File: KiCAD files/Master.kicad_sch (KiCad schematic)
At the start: 24 parts, among them SW1 EG1271A, SW2 EG1271A, SW3 EG1271A, SW4 EG1271A, U4 NUCLEO64-F446RE

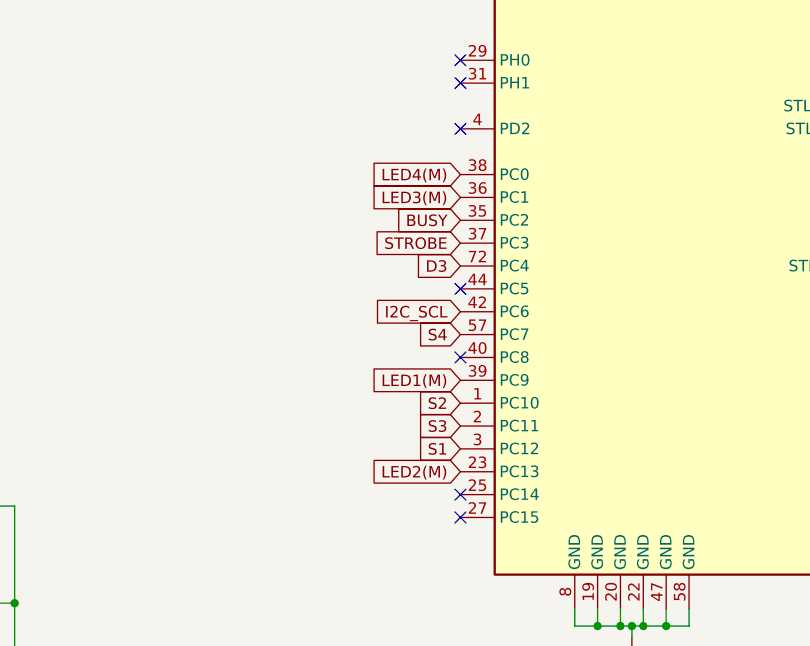
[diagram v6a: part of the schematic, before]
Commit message: update
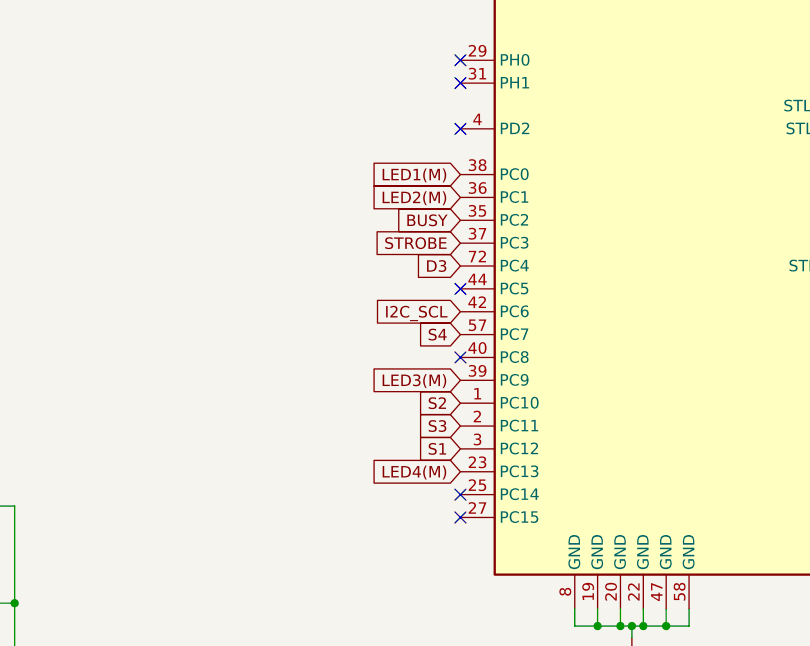
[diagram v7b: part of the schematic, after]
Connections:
- net LED1(M): now also U4.38 (PC0); no longer U4.39 (PC9)
- net LED2(M): now also U4.36 (PC1); no longer U4.23 (PC13)
- net LED3(M): now also U4.39 (PC9); no longer U4.36 (PC1)
- net LED4(M): now also U4.23 (PC13); no longer U4.38 (PC0)
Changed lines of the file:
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@@
     )
   )
-  (global_label "LED1(M)" (shape input) (at 113.665 116.84 180) (fields_autoplaced)
+  (global_label "LED1(M)" (shape input) (at 113.665 93.98 180) (fields_autoplaced)
     (effects (font (size 1.27 1.27)) (justify right))
-    (property "Intersheetrefs" "${INTERSHEET_REFS}" (at 102.8784 116.84 0)
+    (property "Intersheetrefs" "${INTERSHEET_REFS}" (at 102.8784 93.98 0)
       (effects (font (size 1.27 1.27)) (justify right) hide)
     )
   )
-  (global_label "LED3(M)" (shape input) (at 113.665 96.52 180) (fields_autoplaced)
+  (global_label "LED3(M)" (shape input) (at 113.665 116.84 180) (fields_autoplaced)
     (effects (font (size 1.27 1.27)) (justify right))
-    (property "Intersheetrefs" "${INTERSHEET_REFS}" (at 102.8784 96.52 0)
+    (property "Intersheetrefs" "${INTERSHEET_REFS}" (at 102.8784 116.84 0)
       (effects (font (size 1.27 1.27)) (justify right) hide)
     )
@@
     )
   )
-  (global_label "LED4(M)" (shape input) (at 113.665 93.98 180) (fields_autoplaced)
+  (global_label "LED4(M)" (shape input) (at 113.665 127 180) (fields_autoplaced)
     (effects (font (size 1.27 1.27)) (justify right))
-    (property "Intersheetrefs" "${INTERSHEET_REFS}" (at 102.8784 93.98 0)
+    (property "Intersheetrefs" "${INTERSHEET_REFS}" (at 102.8784 127 0)
       (effects (font (size 1.27 1.27)) (justify right) hide)
     )
@@
     )
   )
-  (global_label "LED2(M)" (shape input) (at 113.665 127 180) (fields_autoplaced)
+  (global_label "LED2(M)" (shape input) (at 113.665 96.52 180) (fields_autoplaced)
     (effects (font (size 1.27 1.27)) (justify right))
-    (property "Intersheetrefs" "${INTERSHEET_REFS}" (at 102.8784 127 0)
+    (property "Intersheetrefs" "${INTERSHEET_REFS}" (at 102.8784 96.52 0)
       (effects (font (size 1.27 1.27)) (justify right) hide)
     )

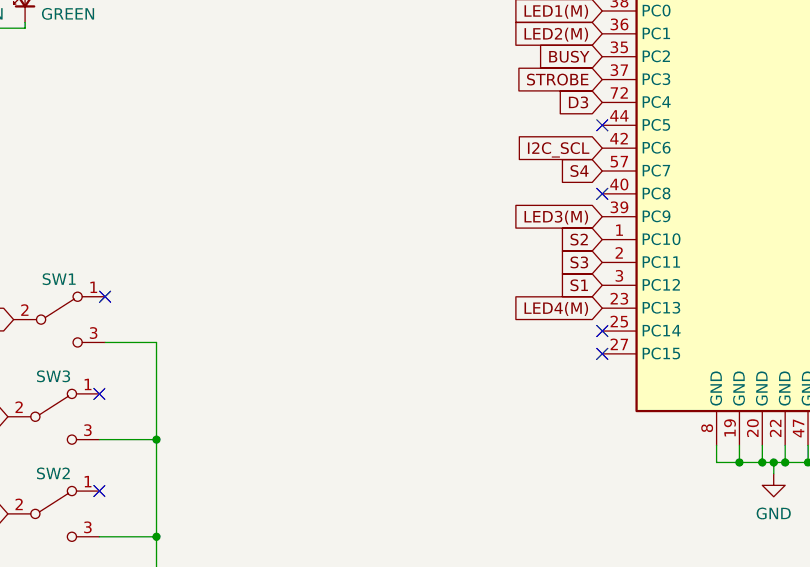
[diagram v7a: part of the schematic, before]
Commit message: update
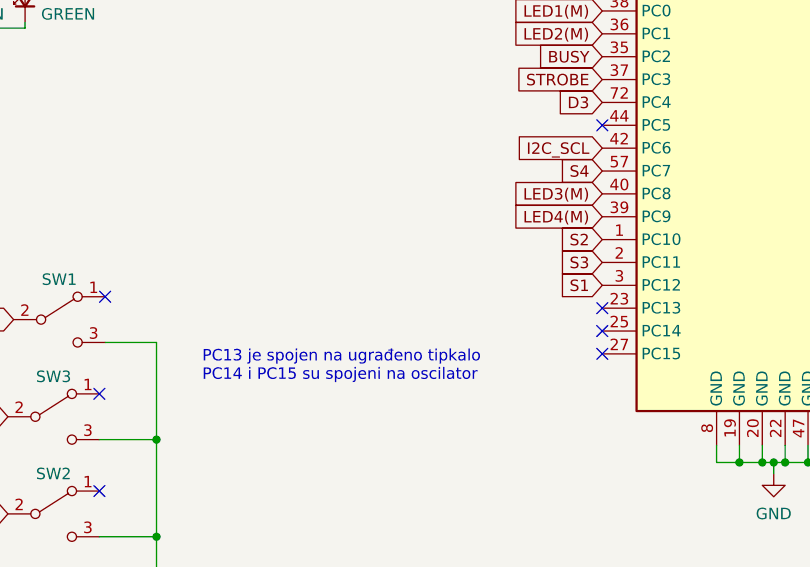
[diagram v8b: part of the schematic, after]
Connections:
- net LED3(M): now also U4.40 (PC8); no longer U4.39 (PC9)
- net LED4(M): now also U4.39 (PC9); no longer U4.23 (PC13)
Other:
- note added: "PC13 je spojen na ugrađeno tipkalo PC14 i PC15 su spojeni na oscilator"
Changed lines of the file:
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@@
   (no_connect (at 169.545 116.84))
   (no_connect (at 113.665 83.82))
+  (no_connect (at 113.665 127))
   (no_connect (at 169.545 88.9))
   (no_connect (at 113.665 129.54))
@@
   (no_connect (at 126.365 40.64))
   (no_connect (at 169.545 86.36))
-  (no_connect (at 113.665 114.3))
   (no_connect (at 141.605 40.64))
   (wire (pts (xy 39.37 43.18) (xy 39.37 43.815))
@@
     (effects (font (size 1.27 1.27)) (justify left bottom))
   )
+  (text "PC13 je spojen na ugrađeno tipkalo\nPC14 i PC15 su spojeni na oscilator"
+    (at 69.215 135.255 0)
+    (effects (font (size 1.27 1.27)) (justify left bottom))
+  )
   (global_label "S3" (shape input) (at 113.665 121.92 180) (fields_autoplaced)
     (effects (font (size 1.27 1.27)) (justify right))
@@
     )
   )
-  (global_label "LED3(M)" (shape input) (at 113.665 116.84 180) (fields_autoplaced)
+  (global_label "LED3(M)" (shape input) (at 113.665 114.3 180) (fields_autoplaced)
+    (effects (font (size 1.27 1.27)) (justify right))
+    (property "Intersheetrefs" "${INTERSHEET_REFS}" (at 102.8784 114.3 0)
+      (effects (font (size 1.27 1.27)) (justify right) hide)
+    )
+  )
+  (global_label "LED4(M)" (shape input) (at 48.895 38.1 90) (fields_autoplaced)
+    (effects (font (size 1.27 1.27)) (justify left))
+    (property "Intersheetrefs" "${INTERSHEET_REFS}" (at 48.895 27.3134 90)
+      (effects (font (size 1.27 1.27)) (justify left) hide)
+    )
+  )
+  (global_label "SPI_MOSI" (shape input) (at 169.545 132.08 0) (fields_autoplaced)
+    (effects (font (size 1.27 1.27)) (justify left))
+    (property "Intersheetrefs" "${INTERSHEET_REFS}" (at 181.1783 132.08 0)
+      (effects (font (size 1.27 1.27)) (justify left) hide)
+    )
+  )
+  (global_label "STROBE" (shape input) (at 113.665 101.6 180) (fields_autoplaced)
+    (effects (font (size 1.27 1.27)) (justify right))
+    (property "Intersheetrefs" "${INTERSHEET_REFS}" (at 103.4832 101.6 0)
+      (effects (font (size 1.27 1.27)) (justify right) hide)
+    )
+  )
+  (global_label "CAN_TD(M)" (shape input) (at 169.545 83.82 0) (fields_autoplaced)
+    (effects (font (size 1.27 1.27)) (justify left))
+    (property "Intersheetrefs" "${INTERSHEET_REFS}" (at 182.5693 83.82 0)
+      (effects (font (size 1.27 1.27)) (justify left) hide)
+    )
+  )
+  (global_label "LED8(M)" (shape input) (at 169.545 76.2 0) (fields_autoplaced)
+    (effects (font (size 1.27 1.27)) (justify left))
+    (property "Intersheetrefs" "${INTERSHEET_REFS}" (at 180.3316 76.2 0)
+      (effects (font (size 1.27 1.27)) (justify left) hide)
+    )
+  )
+  (global_label "LED6(M)" (shape input) (at 169.545 71.12 0) (fields_autoplaced)
+    (effects (font (size 1.27 1.27)) (justify left))
+    (property "Intersheetrefs" "${INTERSHEET_REFS}" (at 180.3316 71.12 0)
+      (effects (font (size 1.27 1.27)) (justify left) hide)
+    )
+  )
+  (global_label "DAC(M)>>ADC(S)" (shape input) (at 107.95 172.085 0) (fields_autoplaced)
+    (effects (font (size 1.27 1.27)) (justify left))
+    (property "Intersheetrefs" "${INTERSHEET_REFS}" (at 127.3849 172.085 0)
+      (effects (font (size 1.27 1.27)) (justify left) hide)
+    )
+  )
+  (global_label "S1" (shape input) (at 48.26 128.27 180) (fields_autoplaced)
+    (effects (font (size 1.27 1.27)) (justify right))
+    (property "Intersheetrefs" "${INTERSHEET_REFS}" (at 42.8558 128.27 0)
+      (effects (font (size 1.27 1.27)) (justify right) hide)
+    )
+  )
+  (global_label "LED5(M)" (shape input) (at 20.955 82.55 90) (fields_autoplaced)
+    (effects (font (size 1.27 1.27)) (justify left))
+    (property "Intersheetrefs" "${INTERSHEET_REFS}" (at 20.955 71.7634 90)
+      (effects (font (size 1.27 1.27)) (justify left) hide)
+    )
+  )
+  (global_label "BUSY" (shape input) (at 113.665 99.06 180) (fields_autoplaced)
+    (effects (font (size 1.27 1.27)) (justify right))
+    (property "Intersheetrefs" "${INTERSHEET_REFS}" (at 105.7812 99.06 0)
+      (effects (font (size 1.27 1.27)) (justify right) hide)
+    )
+  )
+  (global_label "LED1(M)" (shape input) (at 20.32 38.1 90) (fields_autoplaced)
+    (effects (font (size 1.27 1.27)) (justify left))
+    (property "Intersheetrefs" "${INTERSHEET_REFS}" (at 20.32 27.3134 90)
+      (effects (font (size 1.27 1.27)) (justify left) hide)
+    )
+  )
+  (global_label "LED4(M)" (shape input) (at 113.665 116.84 180) (fields_autoplaced)
     (effects (font (size 1.27 1.27)) (justify right))
     (property "Intersheetrefs" "${INTERSHEET_REFS}" (at 102.8784 116.84 0)
       (effects (font (size 1.27 1.27)) (justify right) hide)
     )
-  )
-  (global_label "LED4(M)" (shape input) (at 48.895 38.1 90) (fields_autoplaced)
-    (effects (font (size 1.27 1.27)) (justify left))
-    (property "Intersheetrefs" "${INTERSHEET_REFS}" (at 48.895 27.3134 90)
-      (effects (font (size 1.27 1.27)) (justify left) hide)
-    )
-  )
-  (global_label "SPI_MOSI" (shape input) (at 169.545 132.08 0) (fields_autoplaced)
-    (effects (font (size 1.27 1.27)) (justify left))
-    (property "Intersheetrefs" "${INTERSHEET_REFS}" (at 181.1783 132.08 0)
-      (effects (font (size 1.27 1.27)) (justify left) hide)
-    )
-  )
-  (global_label "STROBE" (shape input) (at 113.665 101.6 180) (fields_autoplaced)
-    (effects (font (size 1.27 1.27)) (justify right))
-    (property "Intersheetrefs" "${INTERSHEET_REFS}" (at 103.4832 101.6 0)
-      (effects (font (size 1.27 1.27)) (justify right) hide)
-    )
-  )
-  (global_label "CAN_TD(M)" (shape input) (at 169.545 83.82 0) (fields_autoplaced)
-    (effects (font (size 1.27 1.27)) (justify left))
-    (property "Intersheetrefs" "${INTERSHEET_REFS}" (at 182.5693 83.82 0)
-      (effects (font (size 1.27 1.27)) (justify left) hide)
-    )
-  )
-  (global_label "LED8(M)" (shape input) (at 169.545 76.2 0) (fields_autoplaced)
-    (effects (font (size 1.27 1.27)) (justify left))
-    (property "Intersheetrefs" "${INTERSHEET_REFS}" (at 180.3316 76.2 0)
-      (effects (font (size 1.27 1.27)) (justify left) hide)
-    )
-  )
-  (global_label "LED6(M)" (shape input) (at 169.545 71.12 0) (fields_autoplaced)
-    (effects (font (size 1.27 1.27)) (justify left))
-    (property "Intersheetrefs" "${INTERSHEET_REFS}" (at 180.3316 71.12 0)
-      (effects (font (size 1.27 1.27)) (justify left) hide)
-    )
-  )
-  (global_label "DAC(M)>>ADC(S)" (shape input) (at 107.95 172.085 0) (fields_autoplaced)
-    (effects (font (size 1.27 1.27)) (justify left))
-    (property "Intersheetrefs" "${INTERSHEET_REFS}" (at 127.3849 172.085 0)
-      (effects (font (size 1.27 1.27)) (justify left) hide)
-    )
-  )
-  (global_label "S1" (shape input) (at 48.26 128.27 180) (fields_autoplaced)
-    (effects (font (size 1.27 1.27)) (justify right))
-    (property "Intersheetrefs" "${INTERSHEET_REFS}" (at 42.8558 128.27 0)
-      (effects (font (size 1.27 1.27)) (justify right) hide)
-    )
-  )
-  (global_label "LED5(M)" (shape input) (at 20.955 82.55 90) (fields_autoplaced)
-    (effects (font (size 1.27 1.27)) (justify left))
-    (property "Intersheetrefs" "${INTERSHEET_REFS}" (at 20.955 71.7634 90)
-      (effects (font (size 1.27 1.27)) (justify left) hide)
-    )
-  )
-  (global_label "BUSY" (shape input) (at 113.665 99.06 180) (fields_autoplaced)
-    (effects (font (size 1.27 1.27)) (justify right))
-    (property "Intersheetrefs" "${INTERSHEET_REFS}" (at 105.7812 99.06 0)
-      (effects (font (size 1.27 1.27)) (justify right) hide)
-    )
-  )
-  (global_label "LED1(M)" (shape input) (at 20.32 38.1 90) (fields_autoplaced)
-    (effects (font (size 1.27 1.27)) (justify left))
-    (property "Intersheetrefs" "${INTERSHEET_REFS}" (at 20.32 27.3134 90)
-      (effects (font (size 1.27 1.27)) (justify left) hide)
-    )
-  )
-  (global_label "LED4(M)" (shape input) (at 113.665 127 180) (fields_autoplaced)
-    (effects (font (size 1.27 1.27)) (justify right))
-    (property "Intersheetrefs" "${INTERSHEET_REFS}" (at 102.8784 127 0)
-      (effects (font (size 1.27 1.27)) (justify right) hide)
-    )
